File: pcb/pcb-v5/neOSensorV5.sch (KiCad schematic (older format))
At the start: 54 parts, among them J1 Conn_01x04, J2 Conn_01x04, J3 Conn_01x05, J4 Conn_01x05, J5 Conn_01x05, J6 Conn_01x03, J7 Conn_01x03, J8 Conn_01x03, J9 Conn_01x03, Q1 2N7002, SW1 clear, SW2 +, SW3 -, U1 HC-SR01, U2 OLED1.3_I2C, U3 ESP32_dev_30p, U4 AMS1117-3.3, U5 LM2902

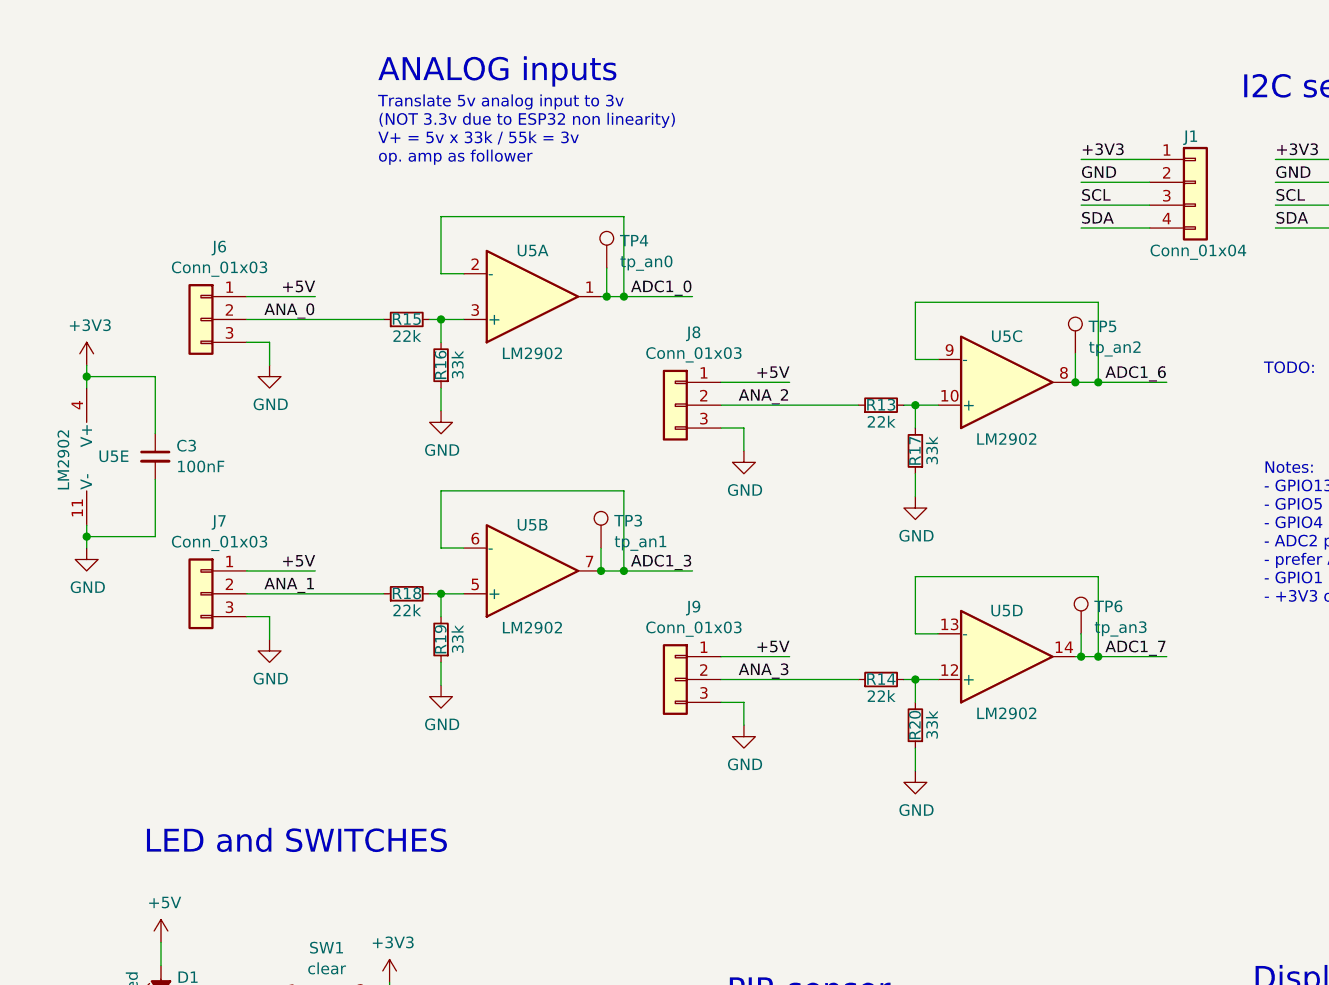
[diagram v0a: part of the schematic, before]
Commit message: update pcb V5
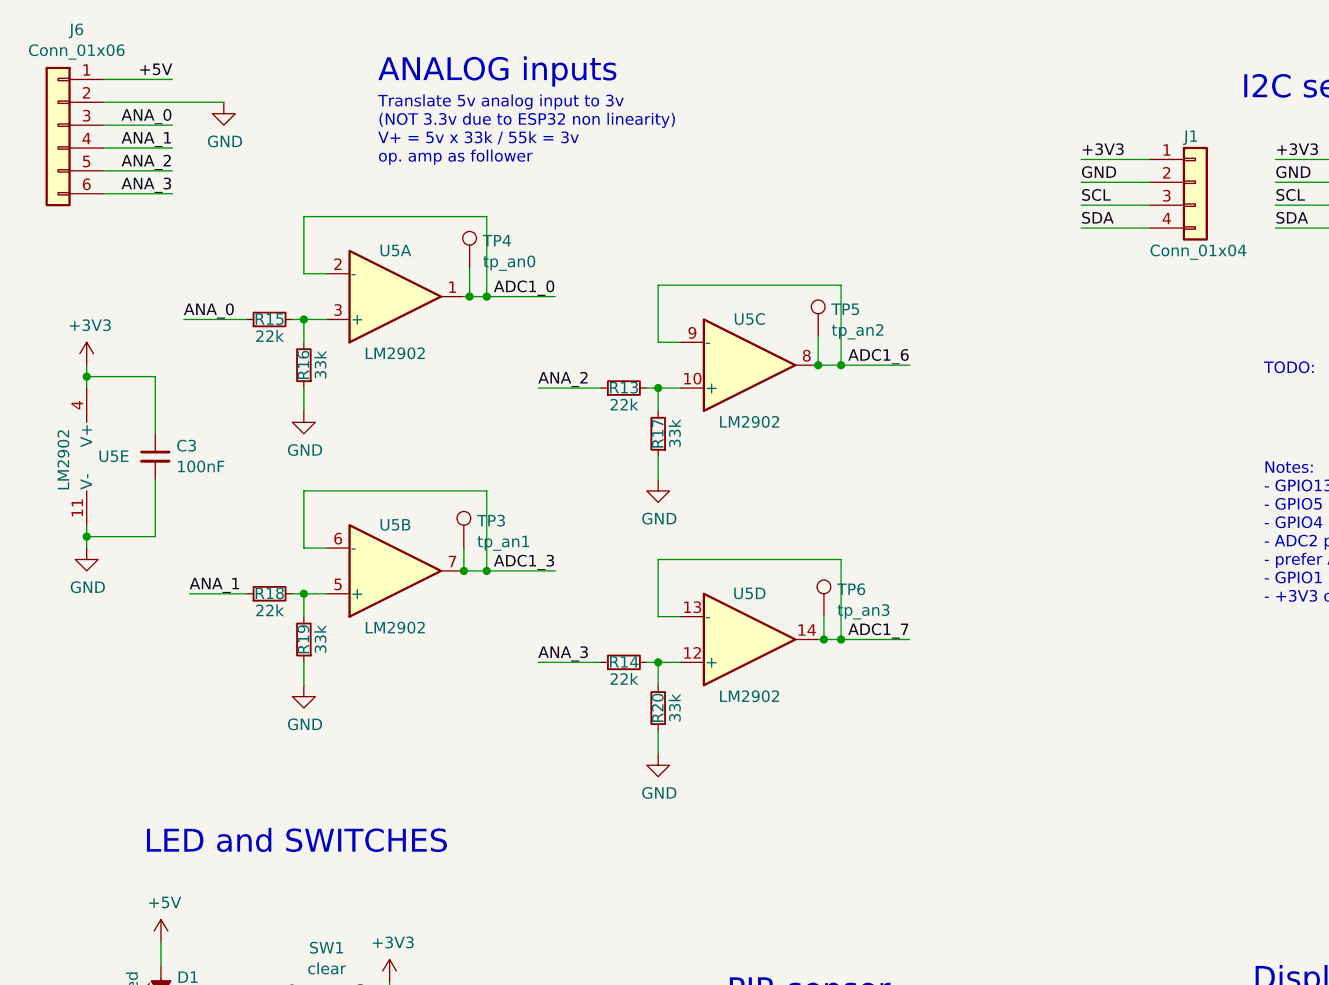
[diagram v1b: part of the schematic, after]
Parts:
- removed J6, J7, J8, J9: Conn_01x03, Connector_PinHeader_2.54mm:PinHeader_1x03_P2.54mm_Vertical, symbol Connector_Generic:Conn_01x03
- added J6: Conn_01x06, Connector_PinHeader_2.54mm:PinHeader_1x06_P2.54mm_Vertical, symbol Connector_Generic:Conn_01x06
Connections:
- net +5V: now also J6.1 (Pin_1)
- net ANA_0: now also J6.3 (Pin_3)
- net ANA_1: now also J6.4 (Pin_4)
- net ANA_2: now also J6.5 (Pin_5)
- net ANA_3: now also J6.6 (Pin_6)
- net GND: now also J6.2 (Pin_2)
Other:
- moved on the sheet: R13, R14, R15, R16, R17, R18, R19, R20, TP3, TP4, TP5, TP6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
